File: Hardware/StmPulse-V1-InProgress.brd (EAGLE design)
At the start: 60.3 x 128.5 mm, 58 parts, among them IC1 78M05, IC2 MCP6004D, U1 MCP6004D, U2-MCP4922 MCP4922MCP4922-SO14

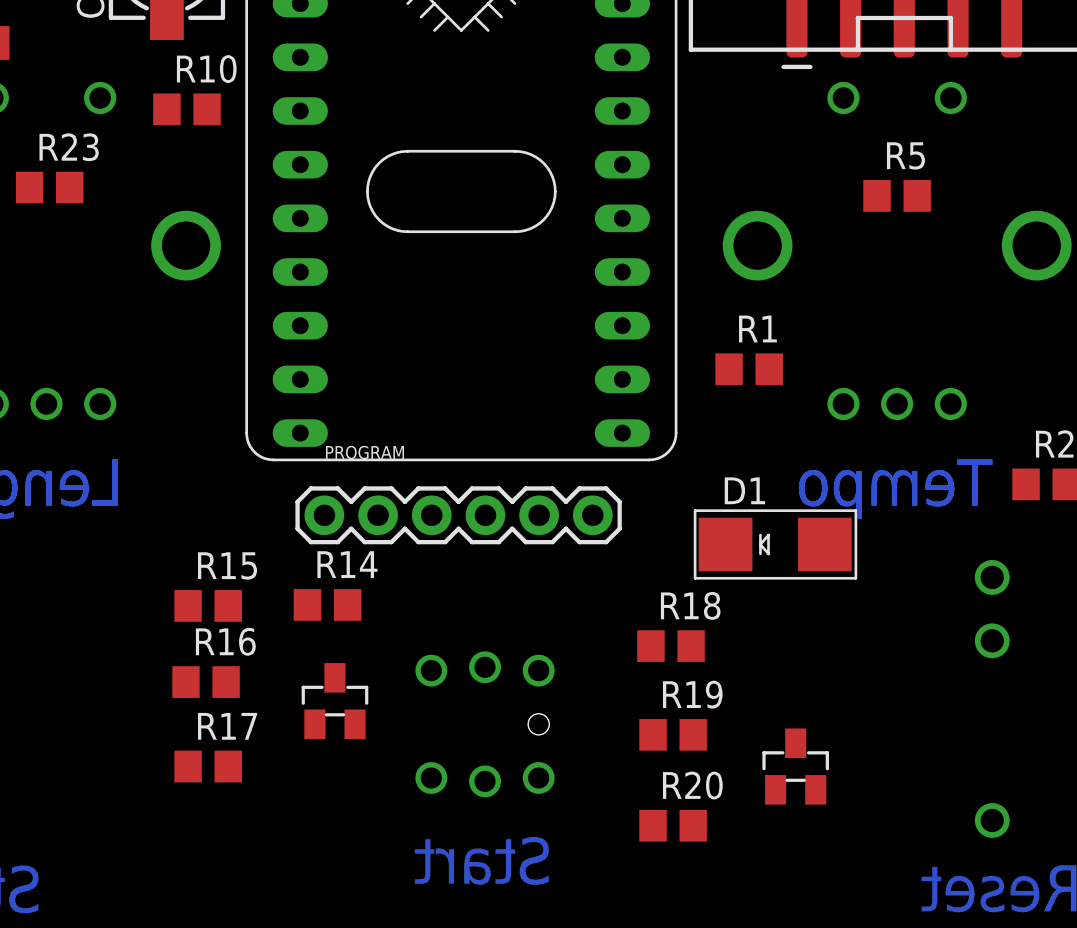
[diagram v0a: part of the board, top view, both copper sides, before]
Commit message: updated hardware
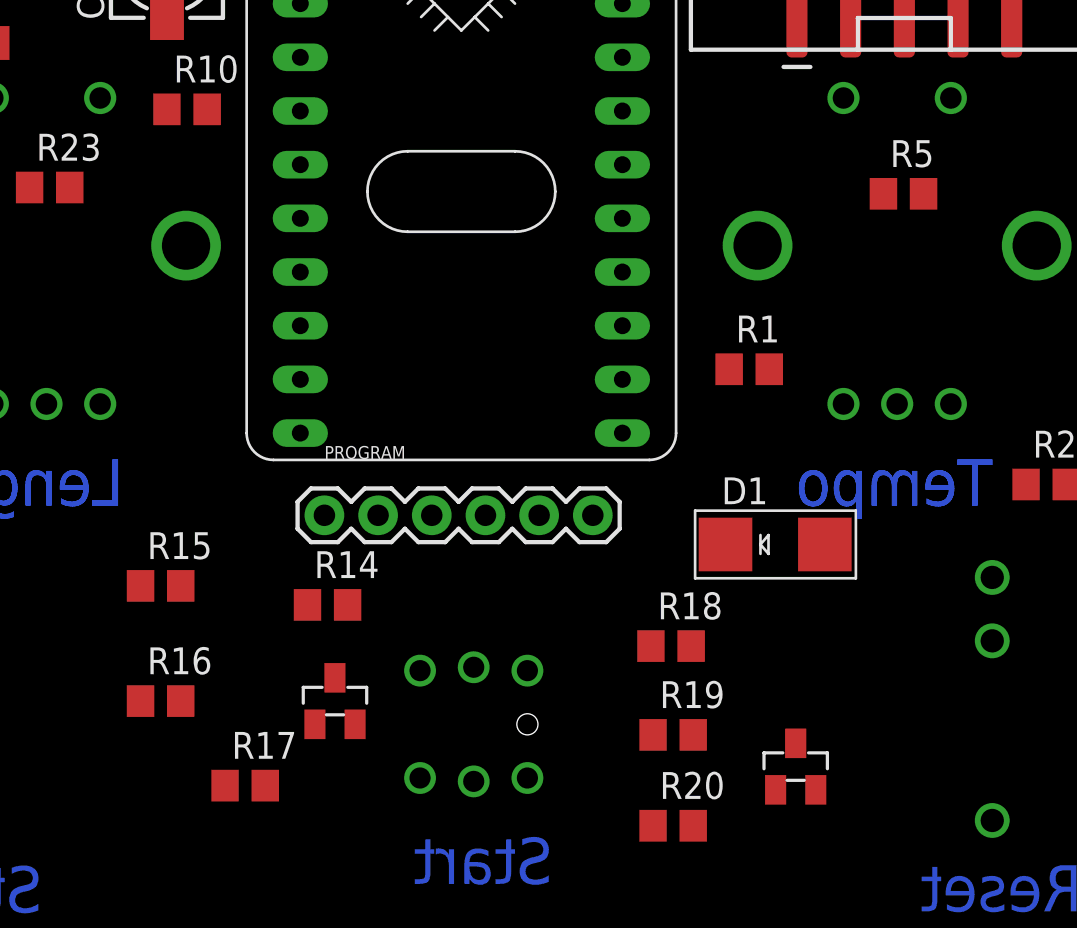
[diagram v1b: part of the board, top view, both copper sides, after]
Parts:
- R14: value 330R -> 220R
- moved R15 2.44 mm to (93.2, -8.90)
- moved R16 2.33 mm to (93.2, -14.3)
- moved R17 1.97 mm to (97.2, -18.4)
- moved BUT3 0.53 mm to (108.1, -15.4)
- moved R5 0.32 mm to (128.4, 9.65)
- renumbered CLOCK to T1_CLOCK, CLOCK1 to T2_RESET
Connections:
- net BUTLED3: now also U$1.P$9; no longer U$1.P$8
